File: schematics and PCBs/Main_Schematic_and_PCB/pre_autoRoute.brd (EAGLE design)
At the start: 88 x 88 mm, 41 parts, among them IC1 LM386N-1, IC2 LM358N

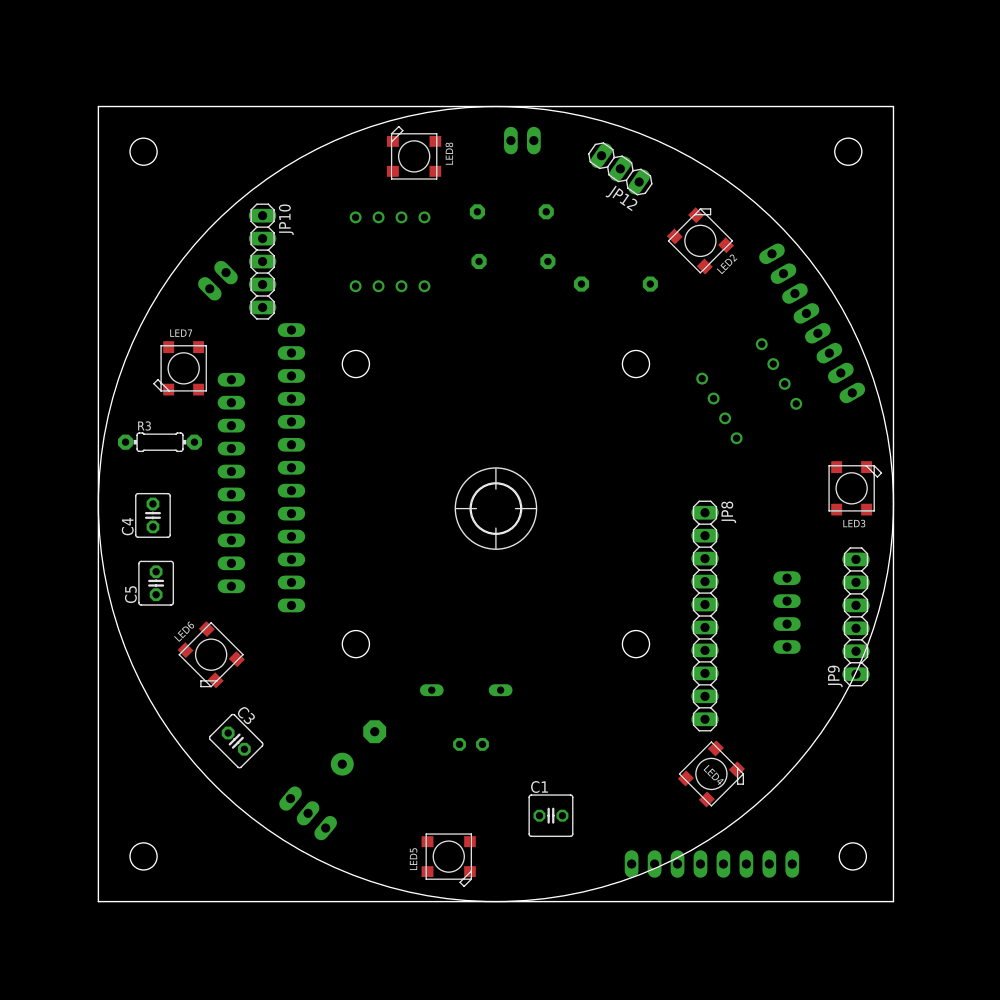
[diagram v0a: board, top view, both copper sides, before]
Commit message: updated main pcb
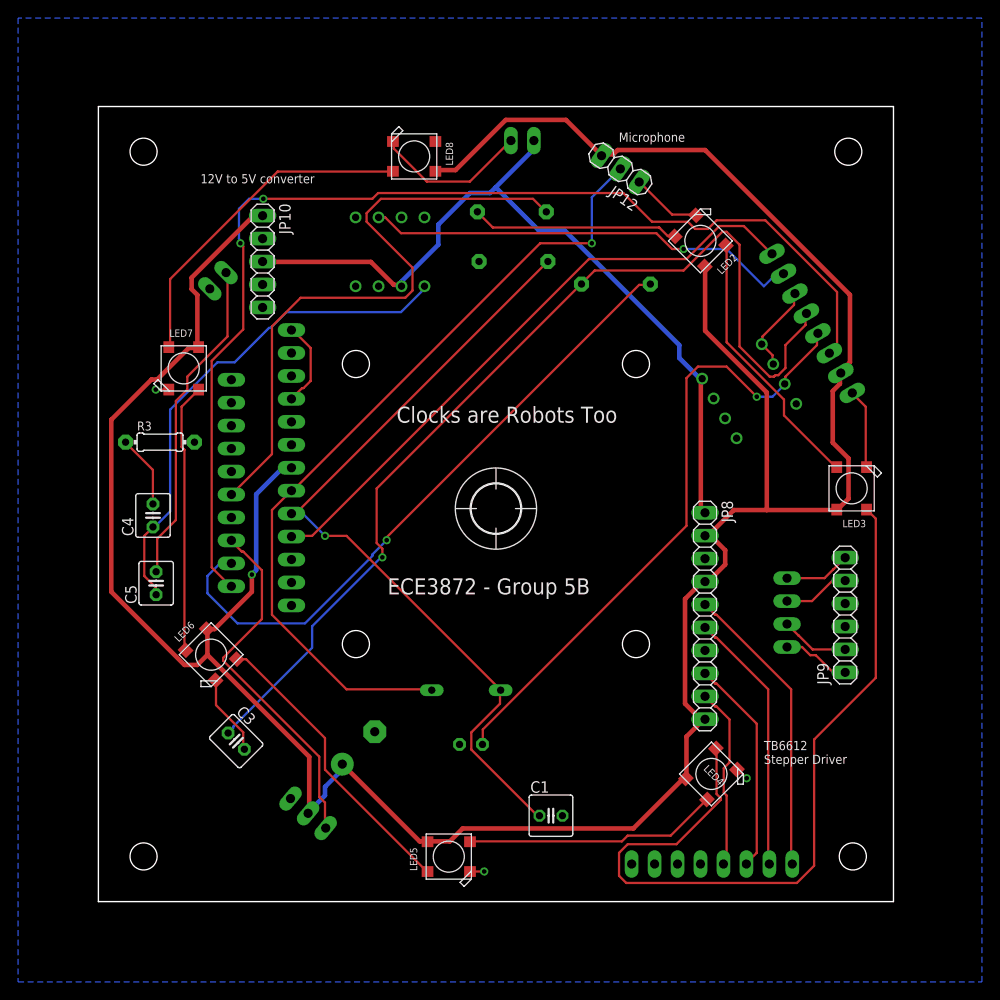
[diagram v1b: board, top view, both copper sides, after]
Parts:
- moved JP9 1.22 mm to (82.7, 31.7)
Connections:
- removed net V+: IC2.8
- removed net V-: IC2.4
- net +12V: now also IC2.8
- net GND: now also IC2.4
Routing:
- net +5V: track 0.00 -> 325.7 mm, vias 0 -> 1
- net D8: track 0.00 -> 123.7 mm, vias 0 -> 2
- net F1: track 0.00 -> 112.2 mm, vias 0 -> 1
- net A0: track 0.00 -> 90.0 mm, vias 0 -> 1
- net A1: track 0.00 -> 89.8 mm, vias 0 -> 1
- net +12V: track 0.00 -> 87.6 mm
- net N$11: track 0.00 -> 87.5 mm
- net D9: track 0.00 -> 71.4 mm, vias 0 -> 1
- net F2: track 0.00 -> 70.5 mm, vias 0 -> 1
- net D12: track 0.00 -> 69.5 mm
- net A2: track 0.00 -> 68.7 mm
- net N$4: track 0.00 -> 56.3 mm
- net AUDIO_OUT_POT: track 0.00 -> 48.6 mm, vias 0 -> 1
- net GND: track 0.00 -> 47.3 mm, vias 0 -> 3
- net D10: track 0.00 -> 39.8 mm
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- added copper zone on layer 16, net GND
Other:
- board text added: "12V to 5V converter"
- board text added: "A0"
- board text added: "A1"
- board text added: "A2"
- board text added: "A3"
- board text added: "Arduino Digital Top"
- board text added: "Arduino Ditial Bottom"
- board text added: "Arduino Power + Analog"
- board text added: "Clocks are Robots Too"
- board text added: "D0"
- board text added: "D1"
- board text added: "D10"
- board text added: "D11"
- board text added: "D12"
- board text added: "D13"
- board text added: "D2"
- board text added: "D3"
- board text added: "D4"
- board text added: "D5"
- board text added: "D6"
- board text added: "D7"
- board text added: "D8"
- board text added: "D9"
- board text added: "ECE3872 - Group 5B"
- board text added: "GND"
- board text added: "Microphone"
- board text added: "MotorA"
- board text added: "MotorB"
- board text added: "Stepper Motor Out"
- board text added: "TB6612 Stepper Driver"
- board text added: "VIN"
